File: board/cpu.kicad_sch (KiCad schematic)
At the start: 6 parts, among them U1 MC68000P

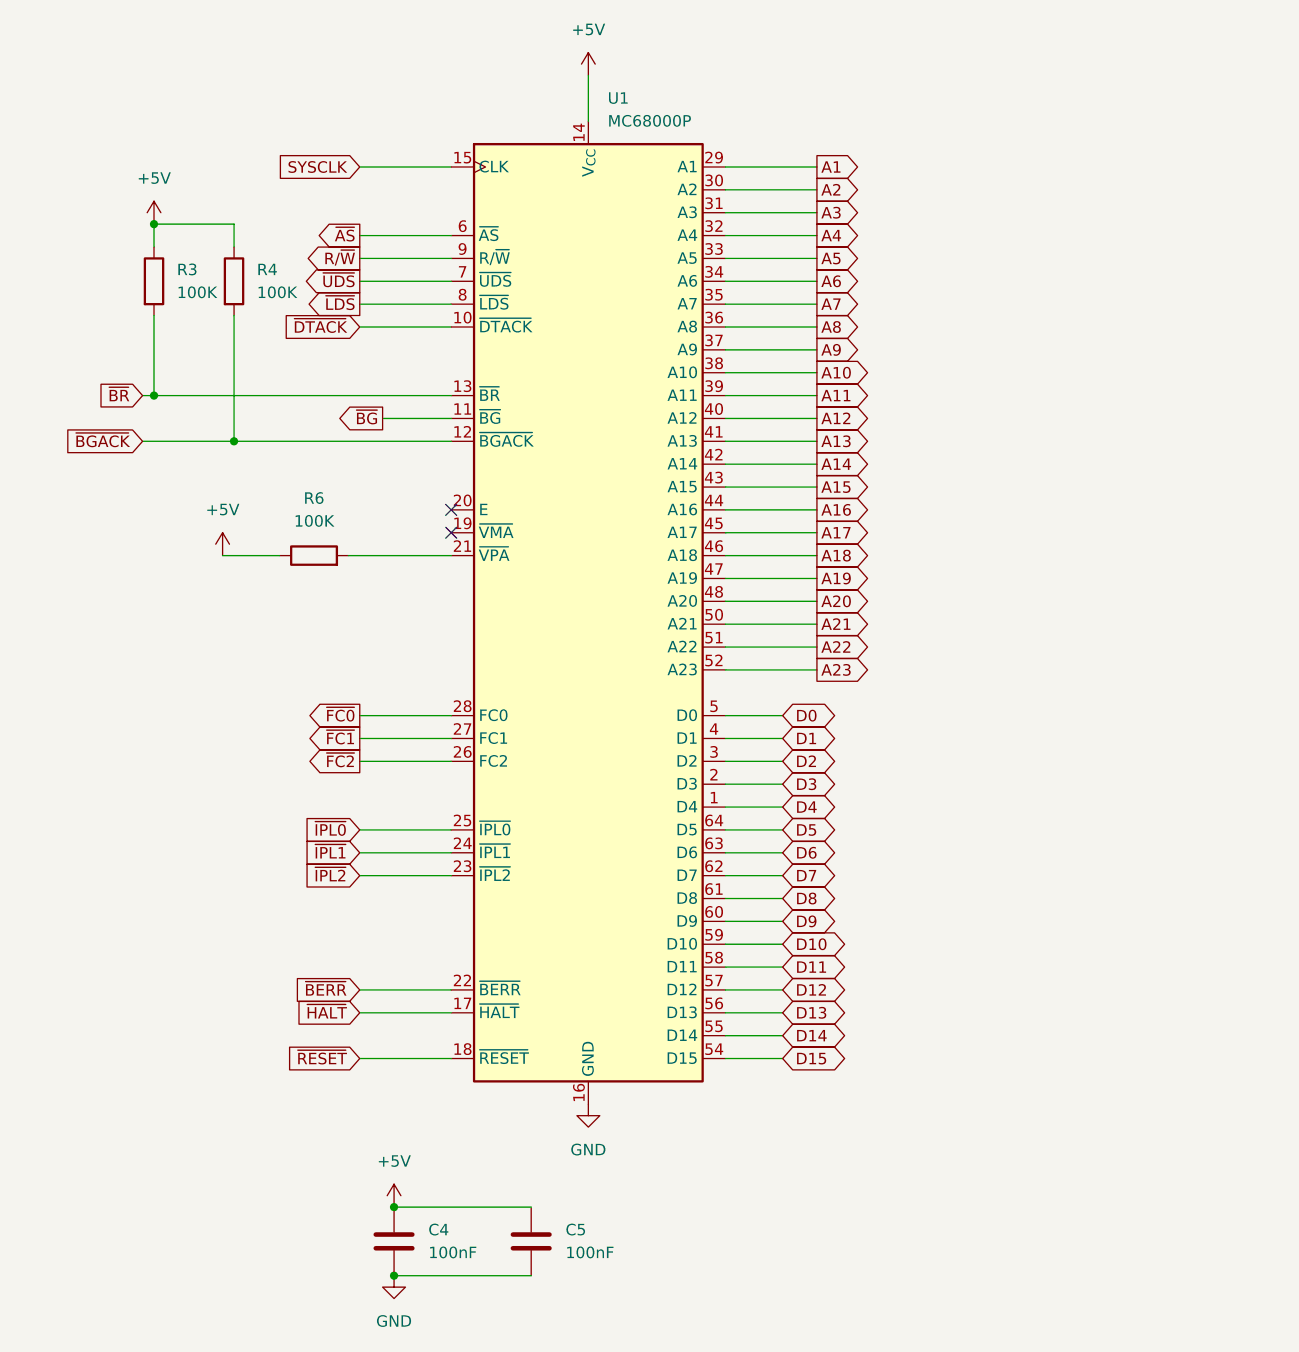
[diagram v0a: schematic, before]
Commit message: design draft complete, added footprints
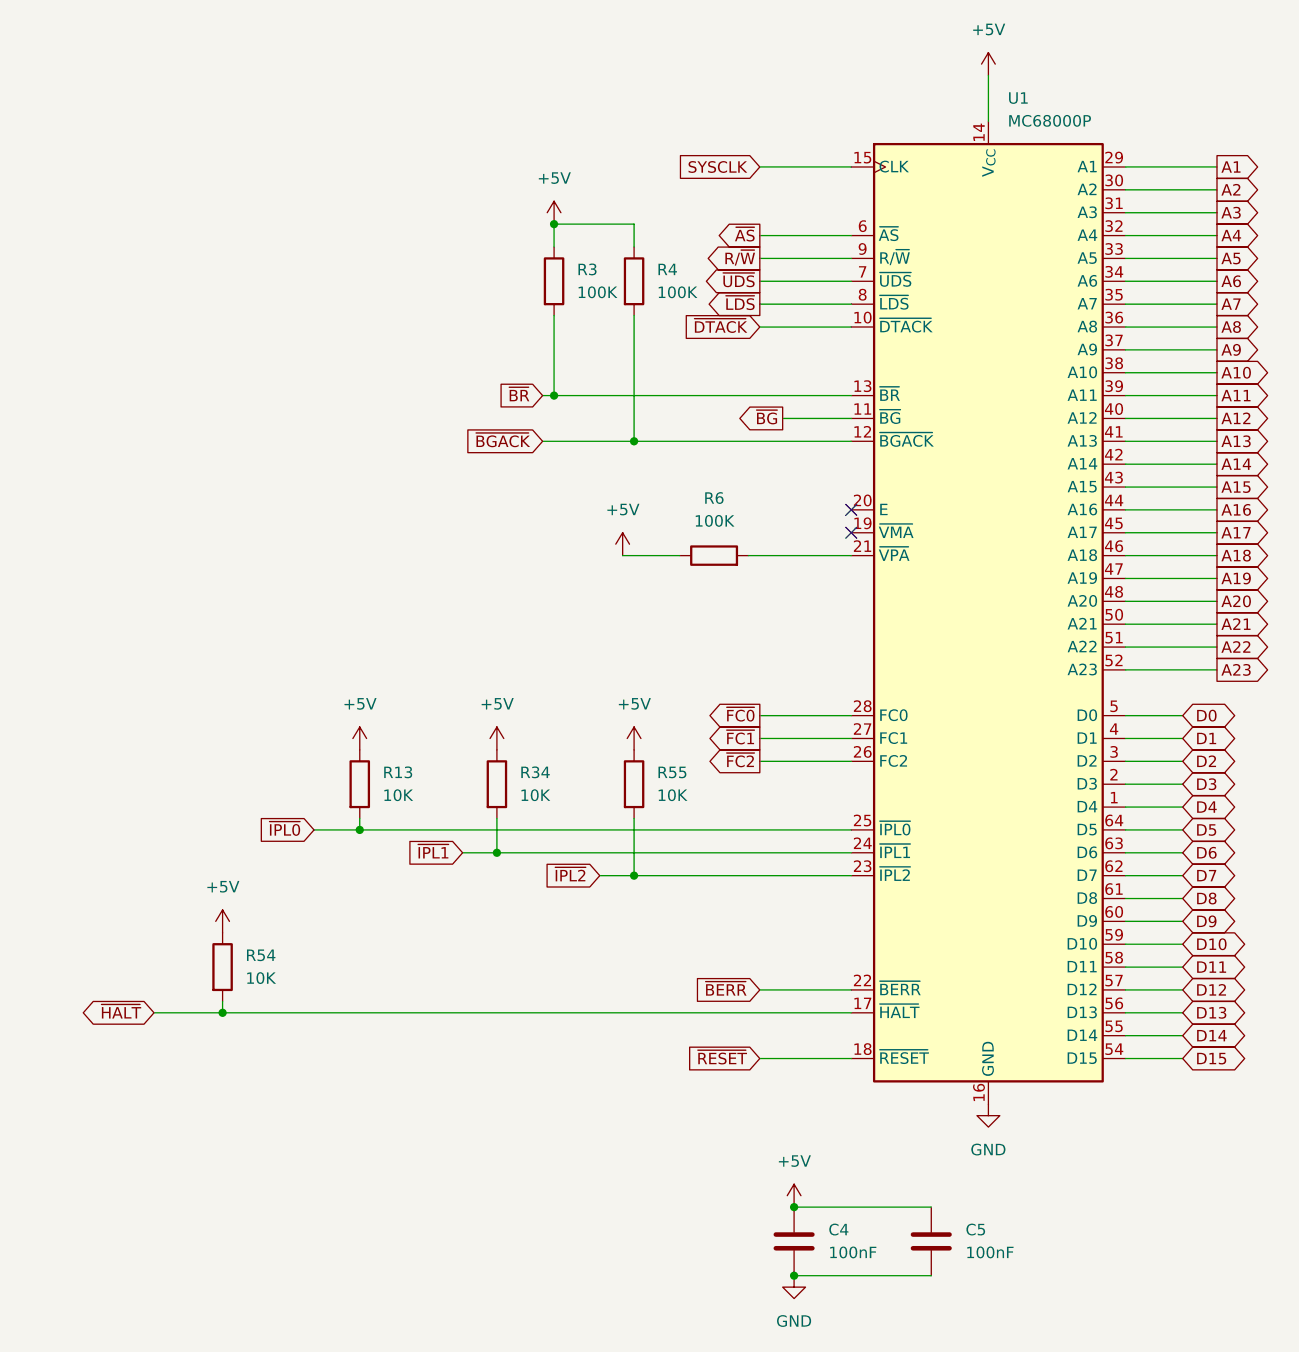
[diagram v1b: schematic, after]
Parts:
- added R13, R34, R54, R55: 10K, Resistor_THT:R_Axial_DIN0207_L6.3mm_D2.5mm_P10.16mm_Horizontal, symbol Device:R
- C4, C5: footprint (none) -> Capacitor_THT:C_Disc_D5.0mm_W2.5mm_P5.00mm
- R3, R4, R6: footprint (none) -> Resistor_THT:R_Axial_DIN0207_L6.3mm_D2.5mm_P10.16mm_Horizontal
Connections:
- net +5V: now also R13.1, R34.1, R54.1, R55.1
- net ~{HALT}: now also R54.2
- net ~{IPL0}: now also R13.2
- net ~{IPL1}: now also R34.2
- net ~{IPL2}: now also R55.2
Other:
- moved on the sheet: C4, C5, R3, R4, R6, U1
